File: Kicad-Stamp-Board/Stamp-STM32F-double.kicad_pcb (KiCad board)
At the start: 2 copper layers, 65 x 84 mm, 70 parts, among them J1 +3.3V, J2 GND, J3 Serial, J4 BOOT1, SW1 Reset, SW2 BOOT, U1 STM32Fxxx, U2 ICL3221, Y1 32.768KHz

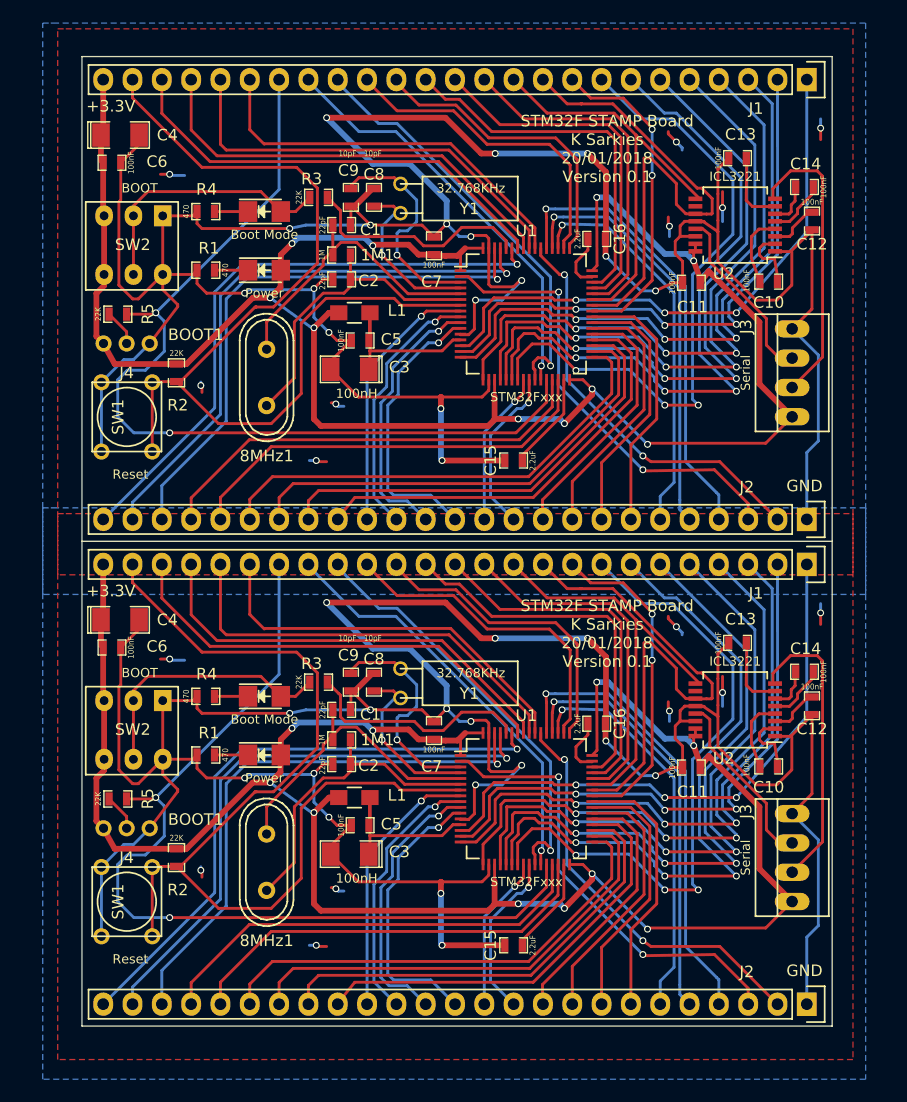
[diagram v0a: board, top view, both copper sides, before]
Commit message: Update PCB to add a jumper on each of pins 48 and 18 to accommodate additional STM32 families.
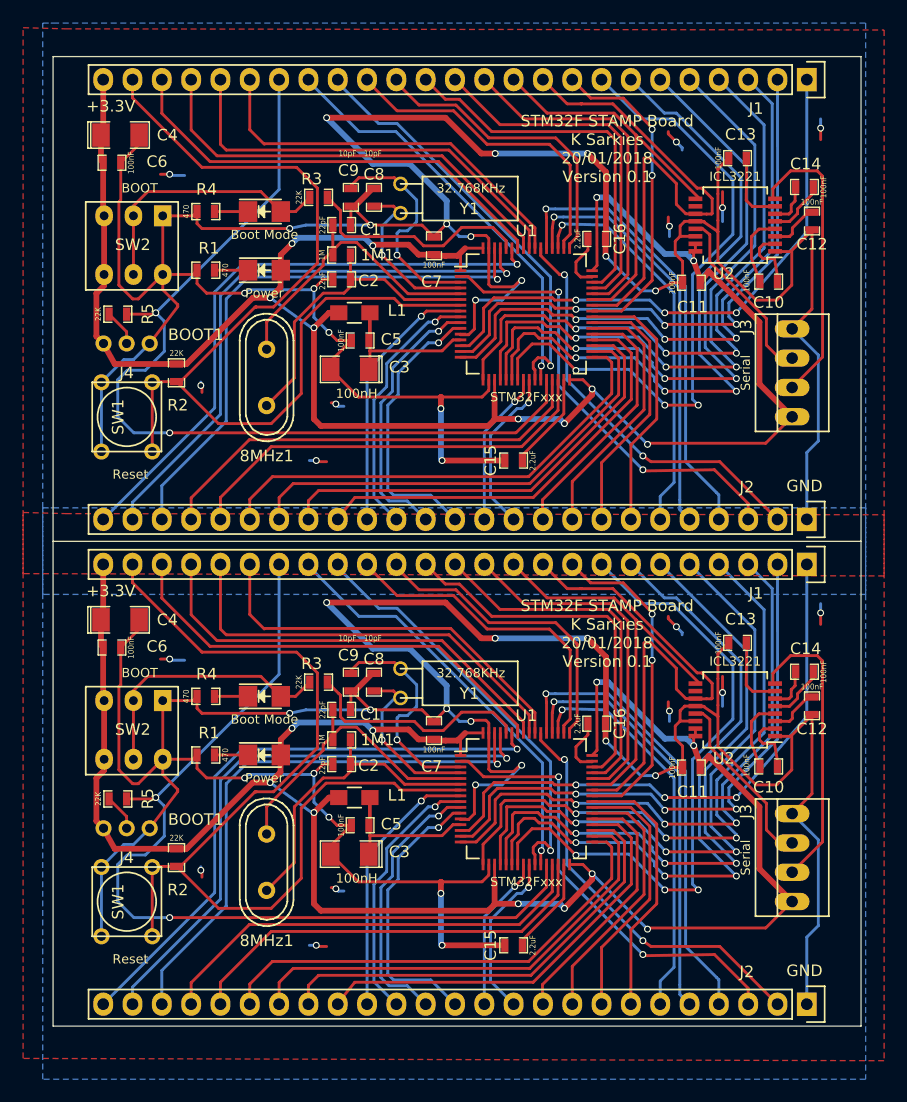
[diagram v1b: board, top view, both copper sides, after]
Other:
- board size 65 x 84 mm -> 70 x 84 mm
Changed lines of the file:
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@@
     (links 331)
     (no_connects 71)
-    (area 111.6 29.3 182.900001 120.800001)
+    (area 109.9 29.3 184.500001 120.800001)
     (thickness 1.6)
     (drawings 7)
@@
       (drillshape 0)
       (scaleselection 1)
-      (outputdirectory gerbers/))
+      (outputdirectory gerbers-x2/))
   )
   (net 0 "")
@@
     )
   )
-  (gr_line (start 115 32.2) (end 180 32.2) (angle 90) (layer Edge.Cuts) (width 0.1))
-  (gr_line (start 180 32.2) (end 180 116.2) (angle 90) (layer Edge.Cuts) (width 0.1))
-  (gr_line (start 115 116.2) (end 115 32.2) (angle 90) (layer Edge.Cuts) (width 0.1))
+  (gr_line (start 112.5 32.2) (end 182.5 32.2) (angle 90) (layer Edge.Cuts) (width 0.1))
+  (gr_line (start 182.5 32.2) (end 182.5 116.2) (angle 90) (layer Edge.Cuts) (width 0.1))
+  (gr_line (start 112.5 116.2) (end 112.5 32.2) (angle 90) (layer Edge.Cuts) (width 0.1))
   (gr_text "STM32F STAMP Board\nK Sarkies\n20/01/2018\nVersion 0.1" (at 160.5 40.2) (layer F.SilkS)
     (effects (font (size 1 1) (thickness 0.2)))
@@
     (effects (font (size 1 1) (thickness 0.2)))
   )
-  (gr_line (start 180 116.2) (end 115 116.2) (angle 90) (layer Edge.Cuts) (width 0.1))
-  (gr_line (start 115 74.2) (end 180 74.2) (angle 90) (layer Edge.Cuts) (width 0.1))
+  (gr_line (start 182.5 116.2) (end 112.5 116.2) (angle 90) (layer Edge.Cuts) (width 0.1))
+  (gr_line (start 112.5 74.2) (end 182.5 74.2) (angle 90) (layer Edge.Cuts) (width 0.1))
   (via (at 170.5 45.3) (size 0.6) (drill 0.4) (layers F.Cu B.Cu) (net 0))
   (segment (start 170.5 45.3) (end 170.5 46.5) (width 0.25) (layer B.Cu) (net 0))
@@
     (polygon
       (pts
-        (xy 113.6 71.8) (xy 181.8 71.8) (xy 181.8 119.1) (xy 112.9 119.1) (xy 112.9 71.8)
+        (xy 113.6 71.8) (xy 184.5 71.9) (xy 184.5 119.2) (xy 109.9 119) (xy 109.9 71.7)
       )
     )
@@
     (polygon
       (pts
-        (xy 113.6 29.8) (xy 181.8 29.8) (xy 181.8 77.1) (xy 112.9 77.1) (xy 112.9 29.8)
+        (xy 113.6 29.8) (xy 184.5 29.9) (xy 184.5 77.2) (xy 109.9 77) (xy 109.9 29.7)
       )
     )

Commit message: Update PCB to stitch grounds a bit more. Update silk screen. Increase length of PCB to 70mm to satisfy fab house requirements.
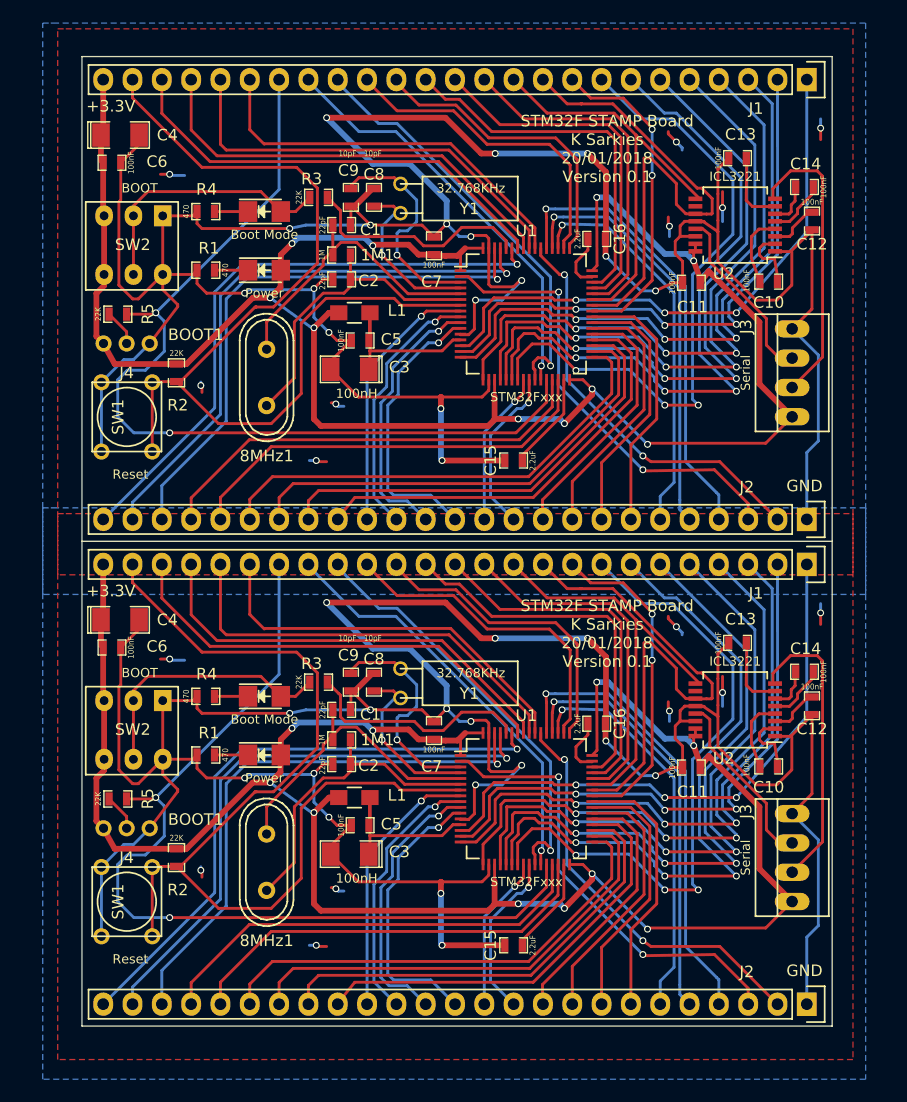
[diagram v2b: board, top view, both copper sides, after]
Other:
- board size 70 x 84 mm -> 65 x 84 mm
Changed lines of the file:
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@@
     (links 331)
     (no_connects 71)
-    (area 109.9 29.3 184.500001 120.800001)
+    (area 111.6 29.3 182.900001 120.800001)
     (thickness 1.6)
     (drawings 7)
@@
       (drillshape 0)
       (scaleselection 1)
-      (outputdirectory gerbers-x2/))
+      (outputdirectory gerbers/))
   )
   (net 0 "")
@@
     )
   )
-  (gr_line (start 112.5 32.2) (end 182.5 32.2) (angle 90) (layer Edge.Cuts) (width 0.1))
-  (gr_line (start 182.5 32.2) (end 182.5 116.2) (angle 90) (layer Edge.Cuts) (width 0.1))
-  (gr_line (start 112.5 116.2) (end 112.5 32.2) (angle 90) (layer Edge.Cuts) (width 0.1))
+  (gr_line (start 115 32.2) (end 180 32.2) (angle 90) (layer Edge.Cuts) (width 0.1))
+  (gr_line (start 180 32.2) (end 180 116.2) (angle 90) (layer Edge.Cuts) (width 0.1))
+  (gr_line (start 115 116.2) (end 115 32.2) (angle 90) (layer Edge.Cuts) (width 0.1))
   (gr_text "STM32F STAMP Board\nK Sarkies\n20/01/2018\nVersion 0.1" (at 160.5 40.2) (layer F.SilkS)
     (effects (font (size 1 1) (thickness 0.2)))
@@
     (effects (font (size 1 1) (thickness 0.2)))
   )
-  (gr_line (start 182.5 116.2) (end 112.5 116.2) (angle 90) (layer Edge.Cuts) (width 0.1))
-  (gr_line (start 112.5 74.2) (end 182.5 74.2) (angle 90) (layer Edge.Cuts) (width 0.1))
+  (gr_line (start 180 116.2) (end 115 116.2) (angle 90) (layer Edge.Cuts) (width 0.1))
+  (gr_line (start 115 74.2) (end 180 74.2) (angle 90) (layer Edge.Cuts) (width 0.1))
   (via (at 170.5 45.3) (size 0.6) (drill 0.4) (layers F.Cu B.Cu) (net 0))
   (segment (start 170.5 45.3) (end 170.5 46.5) (width 0.25) (layer B.Cu) (net 0))
@@
     (polygon
       (pts
-        (xy 113.6 71.8) (xy 184.5 71.9) (xy 184.5 119.2) (xy 109.9 119) (xy 109.9 71.7)
+        (xy 113.6 71.8) (xy 181.8 71.8) (xy 181.8 119.1) (xy 112.9 119.1) (xy 112.9 71.8)
       )
     )
@@
     (polygon
       (pts
-        (xy 113.6 29.8) (xy 184.5 29.9) (xy 184.5 77.2) (xy 109.9 77) (xy 109.9 29.7)
+        (xy 113.6 29.8) (xy 181.8 29.8) (xy 181.8 77.1) (xy 112.9 77.1) (xy 112.9 29.8)
       )
     )
